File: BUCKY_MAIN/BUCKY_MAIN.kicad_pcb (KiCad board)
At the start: 2 copper layers, 156.4 x 156.4 mm, 43 parts, among them IC1 TSSP96038TR, IC10 TSSP96038TR, IC11 TSSP96038TR, IC12 TSSP96038TR, IC2 TSSP96038TR, IC3 TSSP96038TR, IC4 TSSP96038TR, IC5 TSSP96038TR, IC6 TSSP96038TR, IC7 TSSP96038TR, IC8 TSSP96038TR, IC9 TSSP96038TR, J1 Conn_01x10, J2 Conn_01x06, J4 Conn_01x06

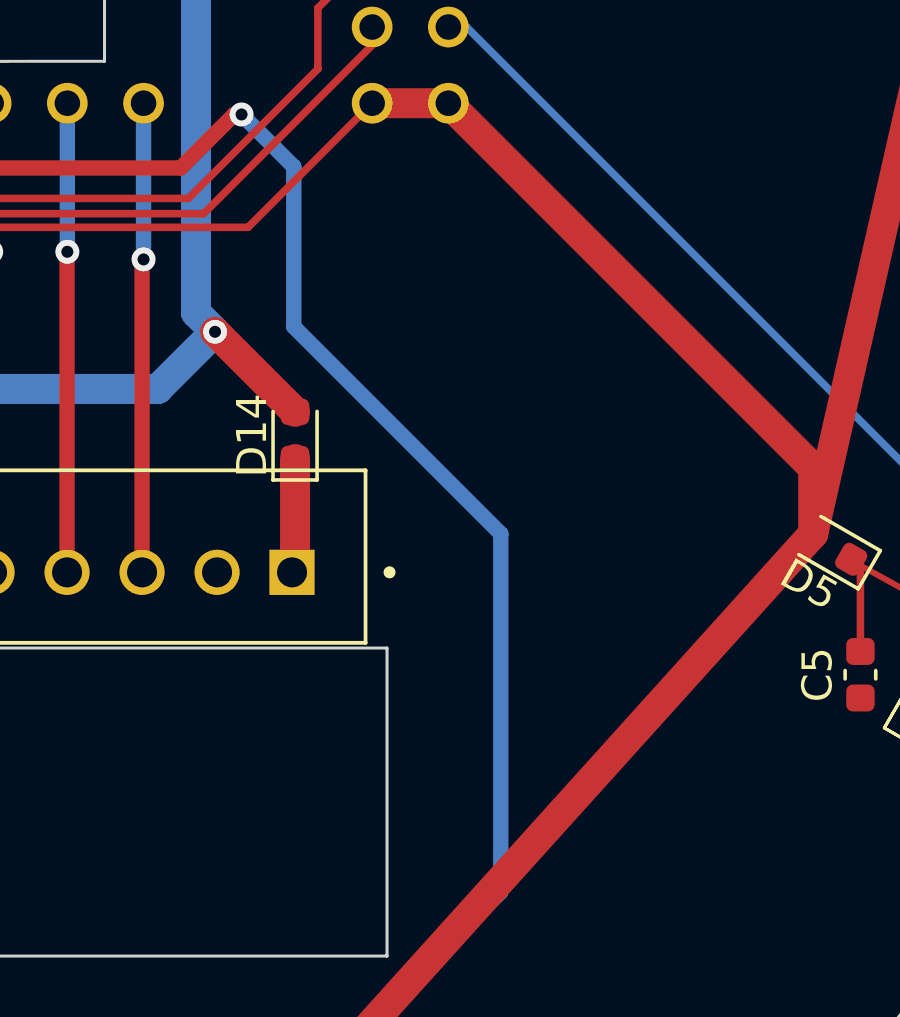
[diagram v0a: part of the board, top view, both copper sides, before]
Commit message: finish up robot (i think)
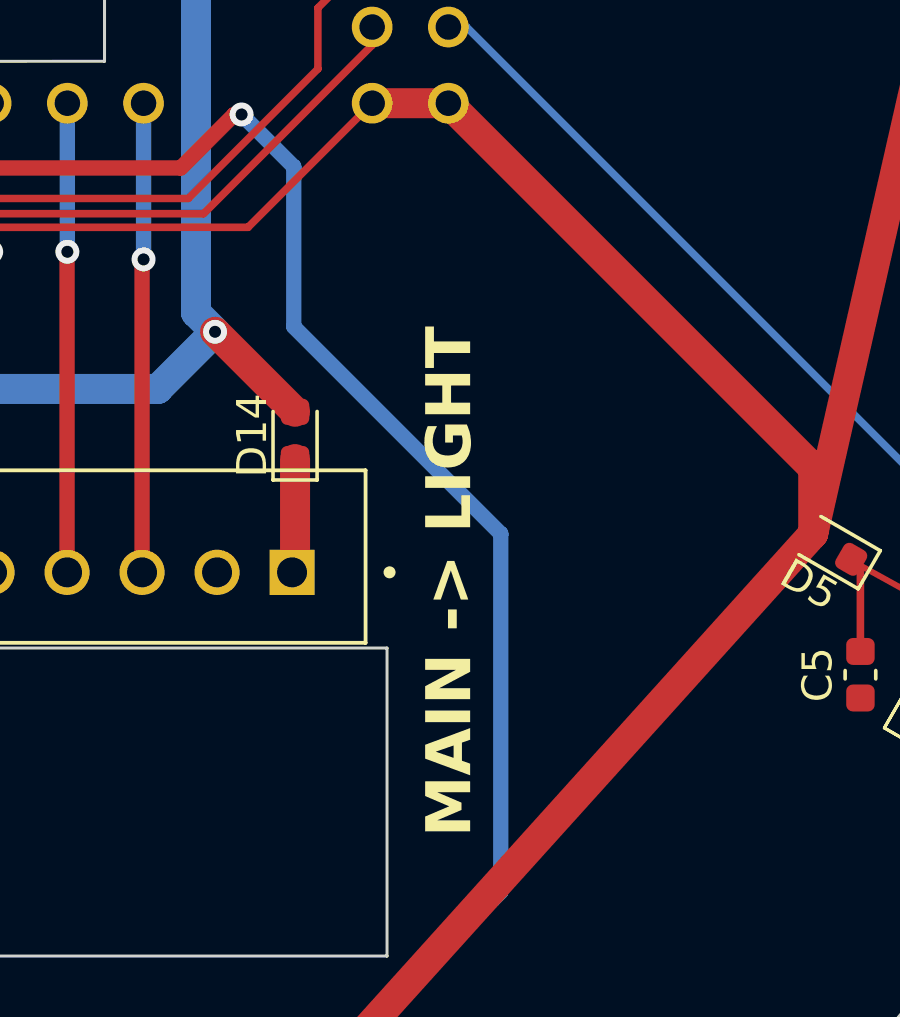
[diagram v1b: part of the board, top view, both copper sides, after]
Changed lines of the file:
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@@
 		(model "${KICAD8_3DMODEL_DIR}/Connector_PinHeader_2.54mm.3dshapes/PinHeader_1x06_P2.54mm_Horizontal.wrl"
 			(offset
-				(xyz 0 0 0)
+				(xyz 0 -12.75 -2)
 			)
 			(scale
@@
 			)
 			(rotate
-				(xyz 0 0 0)
+				(xyz 180 0 0)
 			)
 		)
@@
 		)
 	)
+	(gr_text "MAIN -> LIGHT\n"
+		(at 167.5638 140.9192 90)
+		(layer "F.SilkS")
+		(effects
+			(font
+				(size 1.5 1.5)
+				(thickness 0.3)
+				(bold yes)
+			)
+			(justify left bottom)
+		)
+	)
